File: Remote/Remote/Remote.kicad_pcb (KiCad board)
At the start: 2 copper layers, 46.6 x 70.2 mm, 37 parts, among them J1 USB4125-GF-A_REVA2, J2 B2B-XH-A, J3 61300511121, J4 M20-9990246, U1 MCP73831T-2DCI_OT, U10 DIN, U11 CLK, U12 CS, U13 DC, U14 RST, U15 BL, U2 AP2210N-3.3TRG1, U3 STM32G030F6Px, U4 NRF24L01_Breakout, U5 ADC, U6 VDD, U7 GND, U8 VCC, U9 GND

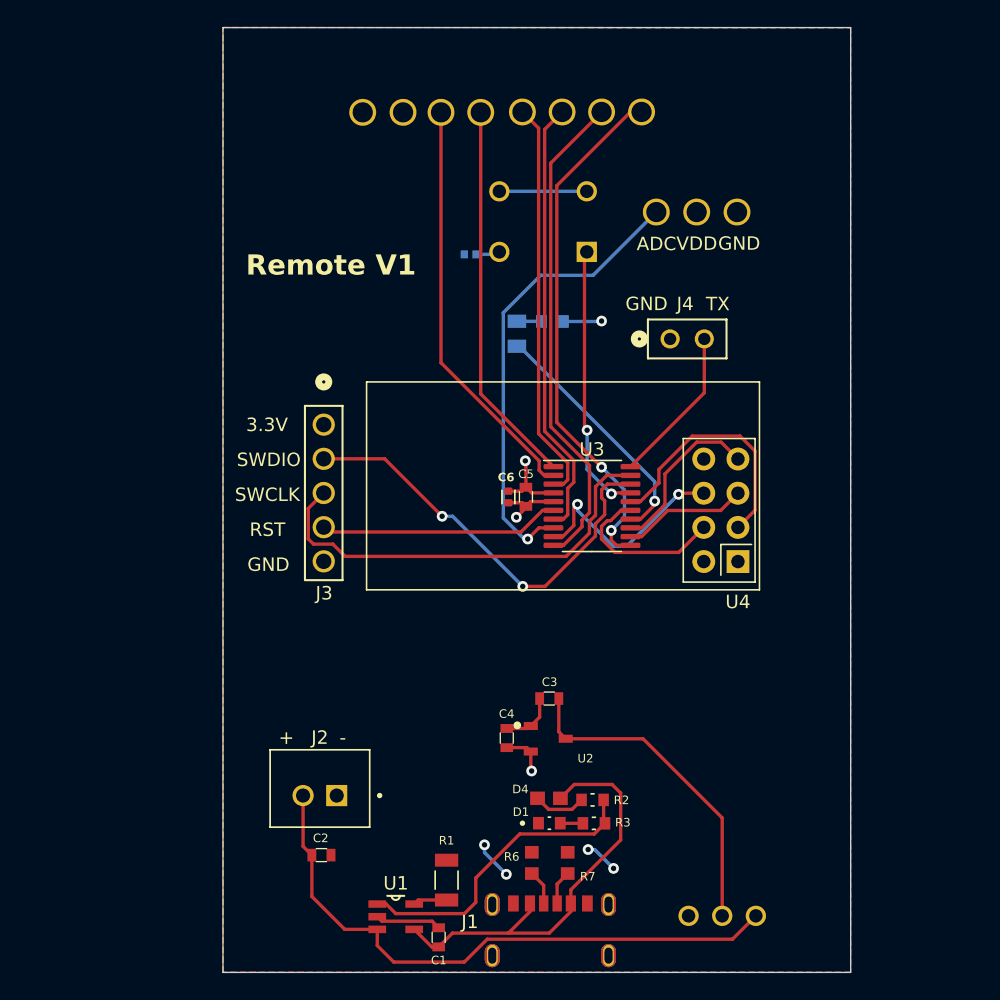
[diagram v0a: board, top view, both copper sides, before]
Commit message: Working sample of the display
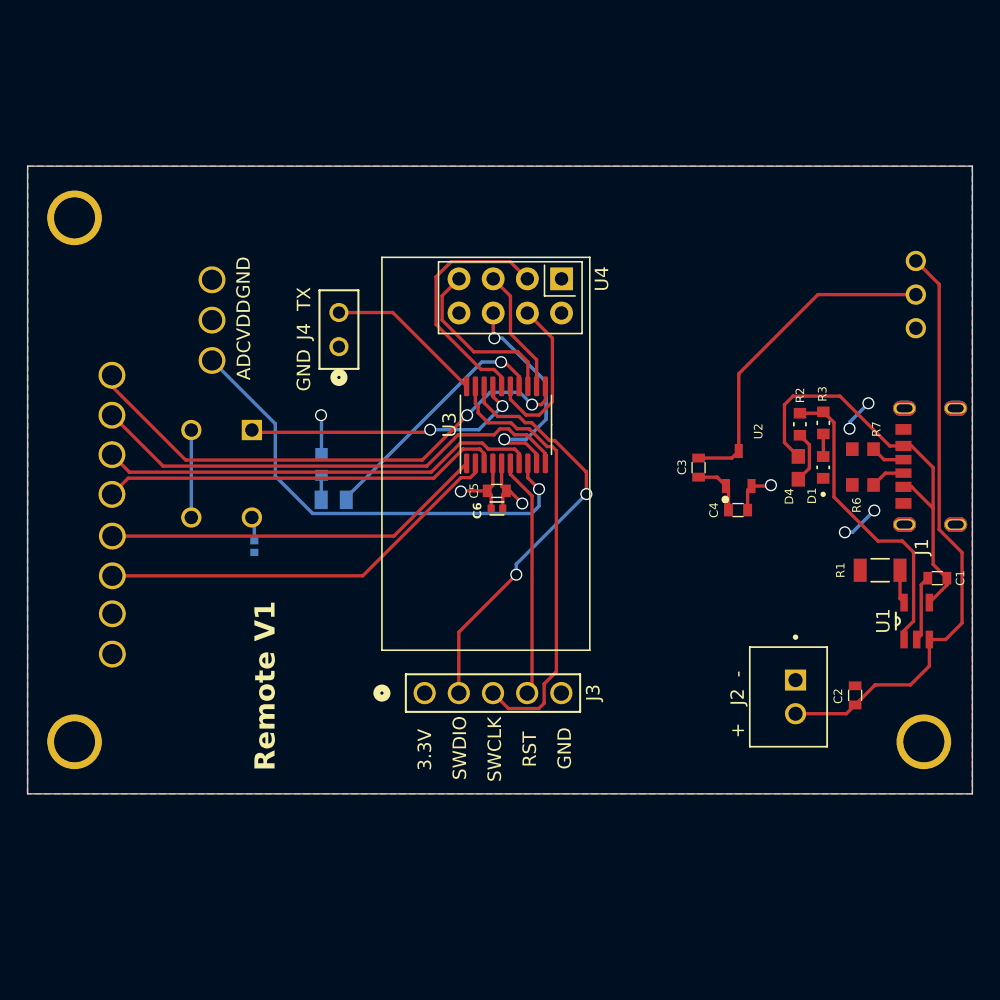
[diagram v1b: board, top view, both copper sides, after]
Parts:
- added ?: , , F.Cu at (110.5, 98.3)
- added ?: , , F.Cu at (110.5, 59.4)
- added ?: , , F.Cu at (173.6, 98.3)
- moved S1 48.4 mm to (173.0, 65.1), turned to -90 degrees
- moved J1 46.1 mm to (175.1, 77.9), turned to 90 degrees
- moved U10 46.0 mm to (113.2, 67.3), turned to 0 degrees
- moved C1 45.7 mm to (174.6, 86.2), turned to 180 degrees
- moved U1 44.5 mm to (173.0, 89.4), turned to 90 degrees
- moved U14 44.3 mm to (113.2, 70.3), turned to 0 degrees
- moved U12 43.5 mm to (113.3, 89.8), turned to 180 degrees
- moved U11 43.1 mm to (113.2, 73.2), turned to 0 degrees
- moved U15 42.4 mm to (113.3, 86.9), turned to 180 degrees
- moved U13 42.2 mm to (113.2, 76.2), turned to 0 degrees
- moved C2 41.4 mm to (168.5, 94.9), turned to -90 degrees
- moved R1 39.6 mm to (170.3, 85.6), turned to 0 degrees
- moved U9 39.3 mm to (117.1, 91.8), turned to -90 degrees
- moved U8 37.9 mm to (117.1, 88.8), turned to -90 degrees
- moved R7 37.8 mm to (169.0, 76.6), turned to 0 degrees
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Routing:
- net /MCU/SPI1_MOSI: track 16.1 -> 17.2 mm
- net /MCU/Button: track 20.3 -> 21.3 mm
- net /MCU/ADC1_IN1: track 34.4 -> 35.0 mm
- net /MCU/SPI1_MISO: track 12.5 -> 13.1 mm
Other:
- board size 46.6 x 70.2 mm -> 70.2 x 46.7 mm
